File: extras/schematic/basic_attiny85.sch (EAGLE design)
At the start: 9 parts, among them U2 ATTINY85-20P

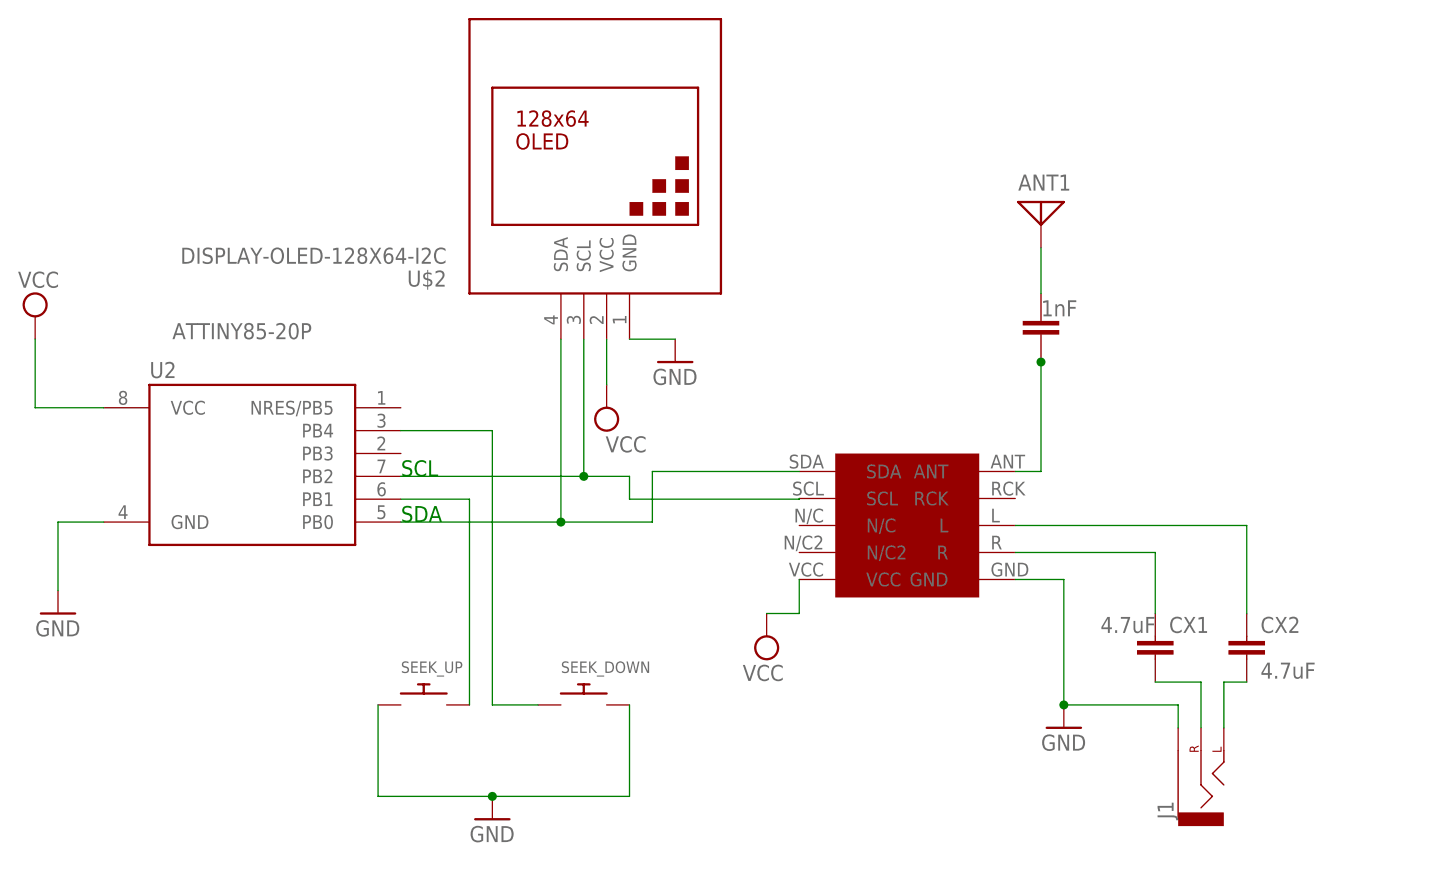
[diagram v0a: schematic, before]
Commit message: RDA5807 Arduino Library
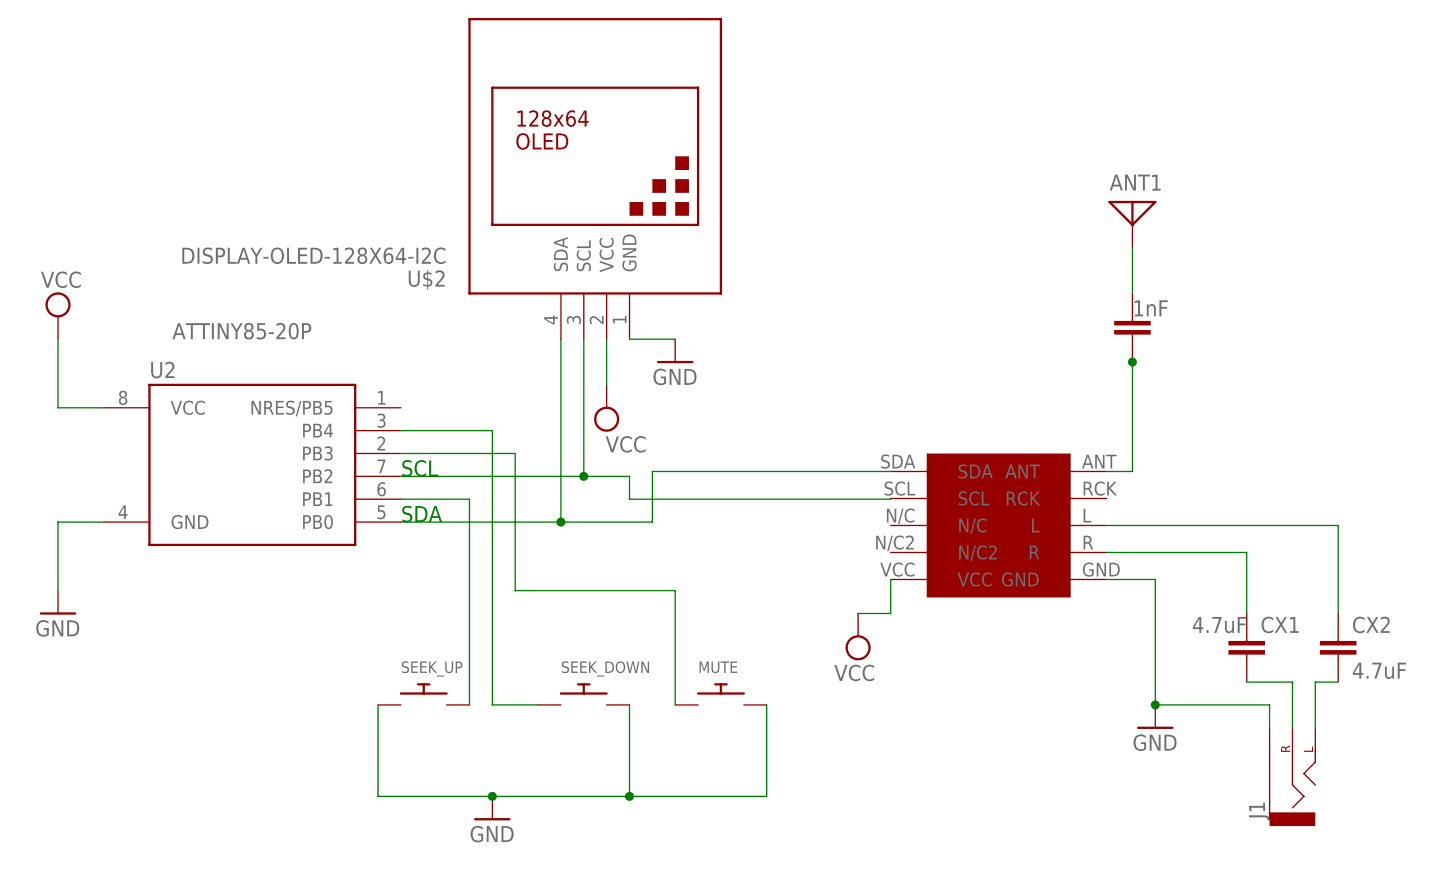
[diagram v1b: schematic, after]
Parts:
- added MUTE: (no value), adafruit:SWITCH_PUSHBUTTONC&K_KSS
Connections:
- new net N$3: MUTE.P$1, U2.PB3
- net GND: now also MUTE.P$2
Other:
- moved on the sheet: ANT1, CX1, CX2, J1
